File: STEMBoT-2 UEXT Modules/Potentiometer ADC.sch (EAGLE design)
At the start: 19 parts, among them IC1 74HC165PW,118, IC2 LMV324DR2G, IC3 LMV324DR2G, Q1 MMBT3904LP-7, U1 SN74HC148D

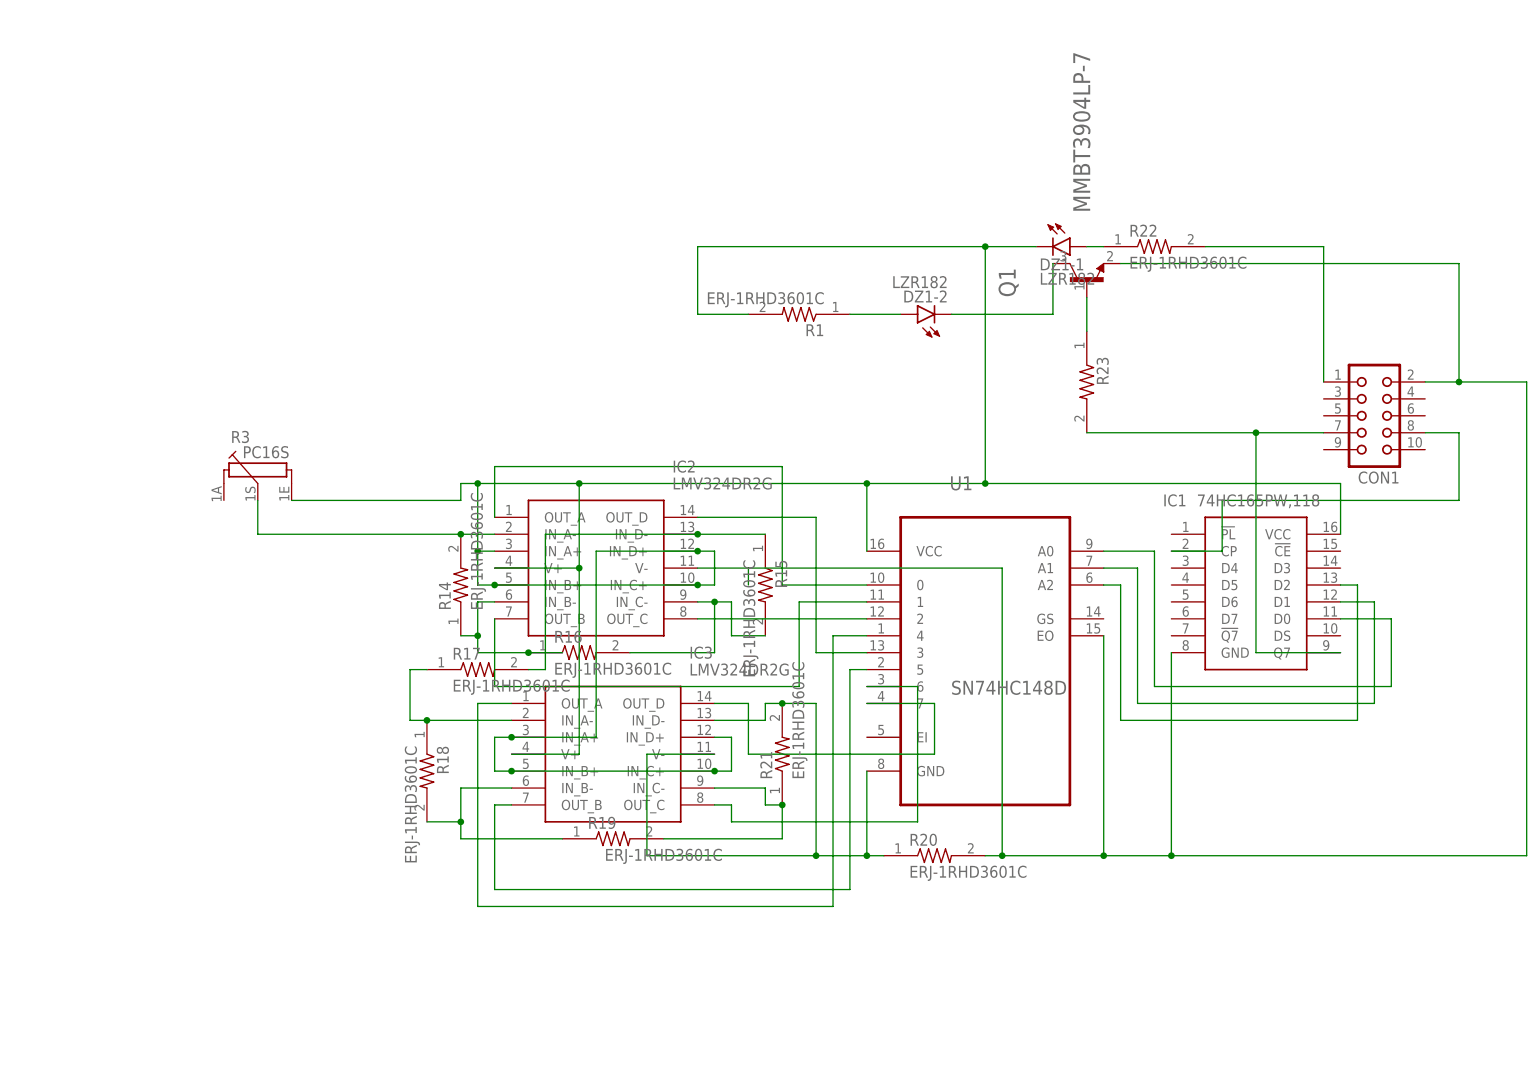
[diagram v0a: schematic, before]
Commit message: Once again, updating ADC shematics and boards. Used autorouter.
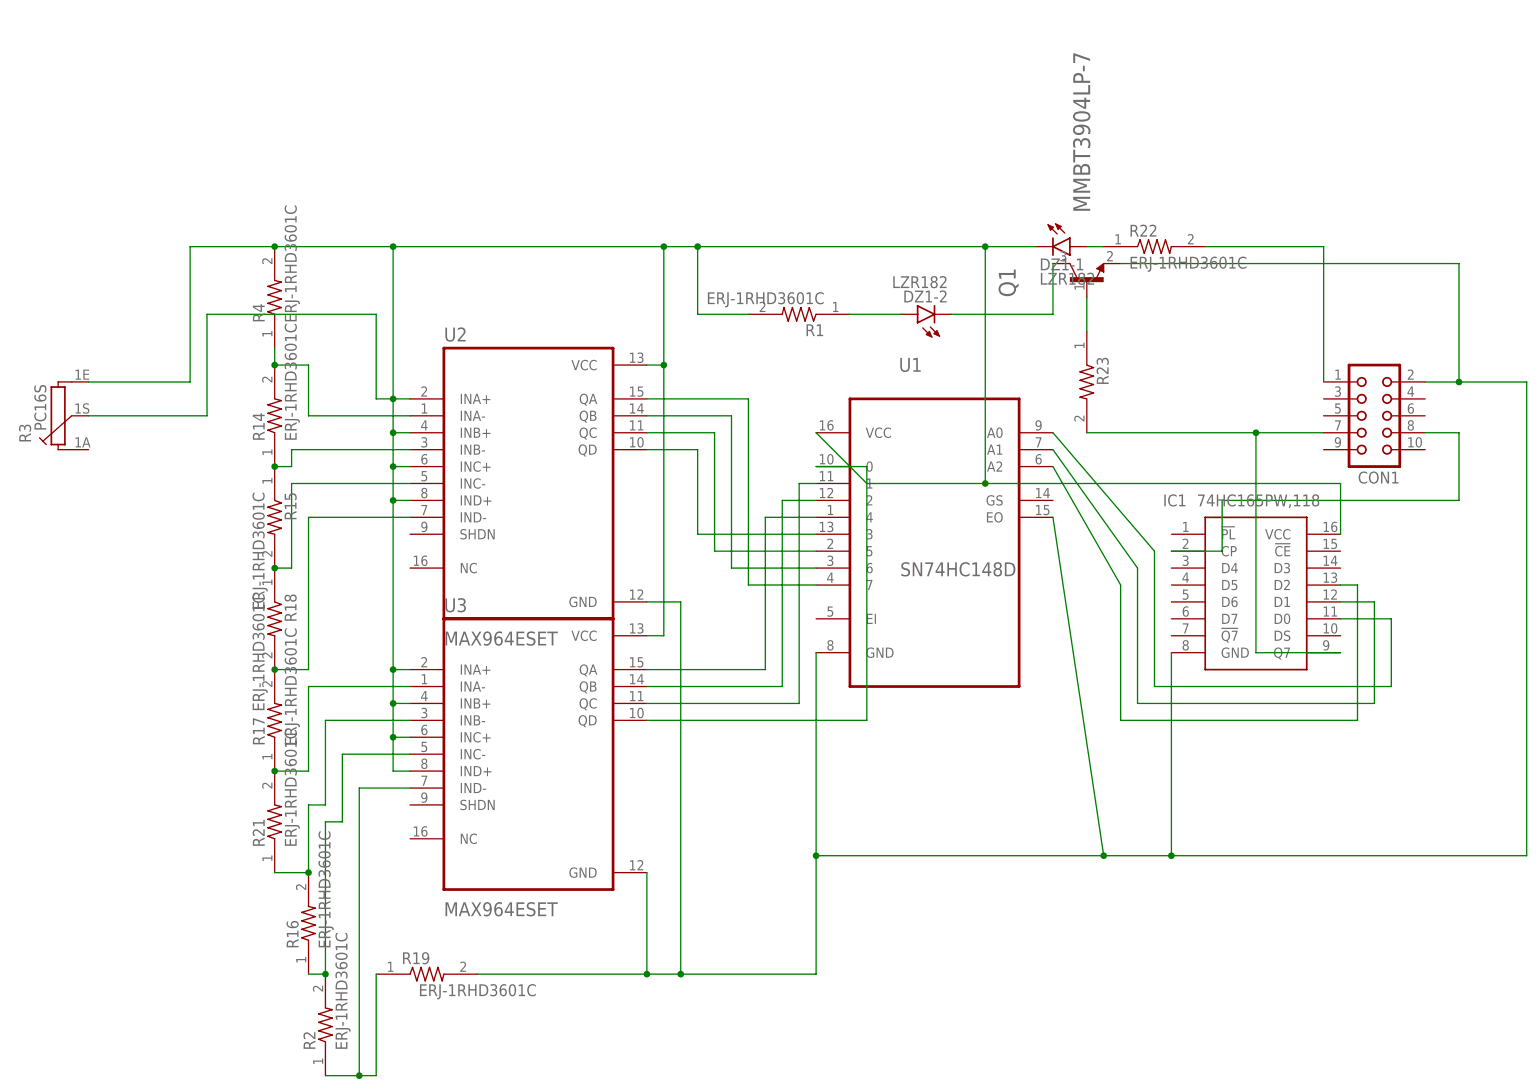
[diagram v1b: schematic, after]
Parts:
- removed IC2, IC3: LMV324DR2G, LMV324DR2G:LMV324DR2G
- removed R20: ERJ-1RHD3601C, Resistor:ERJ-1RHD3601C
- added R2, R4: ERJ-1RHD3601C, Resistor:ERJ-1RHD3601C
- added U2, U3: MAX964ESET, MAX964ESET:MAX964ESET
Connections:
- removed net N$17: IC3.IN_C-, R19.2, R21.1
- removed net N$31: IC2.OUT_C, U1.2
- removed net N$32: IC2.OUT_B, U1.1
- removed net N$33: IC2.OUT_A, U1.0
- removed net N$5: DZ1-1.C, IC1.VCC, IC2.IN_A+, IC2.IN_B+, IC2.IN_C+, IC2.IN_D+, IC2.V+, IC3.IN_A+, IC3.IN_B+, IC3.IN_C+, IC3.IN_D+, IC3.V+, R1.2, R3.1E, U1.VCC
- new net N$21: U1.5, U2.QC
- new net N$27: U1.2, U3.QB
- new net N$28: U1.1, U3.QC
- new net N$29: U1.0, U3.QD
- new net N$30: DZ1-1.C, IC1.VCC, R1.2, R3.1E, R3.1S, R4.2, U1.VCC, U2.INA+, U2.INB+, U2.INC+, U2.IND+, U2.VCC, U3.INA+, U3.INB+, U3.INC+, U3.IND+, U3.VCC
- net N$1: now also R16.1, R2.2, U3.INC-; no longer IC3.IN_D-, IC3.V-, R20.1, R21.2, U1.GND
- net N$10: now also R16.2, R21.1, U3.INB-; no longer IC2.IN_B-, R14.1, R16.1
- net N$11: now also R19.1, R2.1, U3.IND-; no longer IC2.IN_A-, R14.2, R3.1S
- net N$12: now also R19.2, U1.GND, U2.GND, U3.GND; no longer IC2.V-, R20.2
- net N$13: now also U1.7, U2.QA; no longer IC2.IN_C-, R15.2, R16.2
- net N$14: now also U1.6, U2.QB; no longer IC2.IN_D-, R15.1, R17.2
- net N$23: now also U1.3, U2.QD; no longer IC3.OUT_B, U1.5
- net N$26: now also U3.QA; no longer IC3.OUT_A
- net N$3: now also R14.2, R4.1, U2.INA-; no longer IC3.IN_A-, R17.1, R18.1
- net N$4: now also R14.1, R15.1, U2.INB-; no longer IC2.OUT_D, U1.3
- net N$6: now also R15.2, R18.1, U2.INC-; no longer IC3.OUT_C, U1.6
- net N$7: now also R17.2, R18.2, U2.IND-; no longer IC3.OUT_D, U1.7
- net N$9: now also R17.1, R21.2, U3.INA-; no longer IC3.IN_B-, R18.2, R19.1
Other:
- moved on the sheet: R14, R15, R16, R17, R18, R19, R21, R3, U1
